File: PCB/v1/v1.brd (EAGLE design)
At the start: 55 x 39 mm, 69 parts, among them U2 AT24C512C-SHD-B

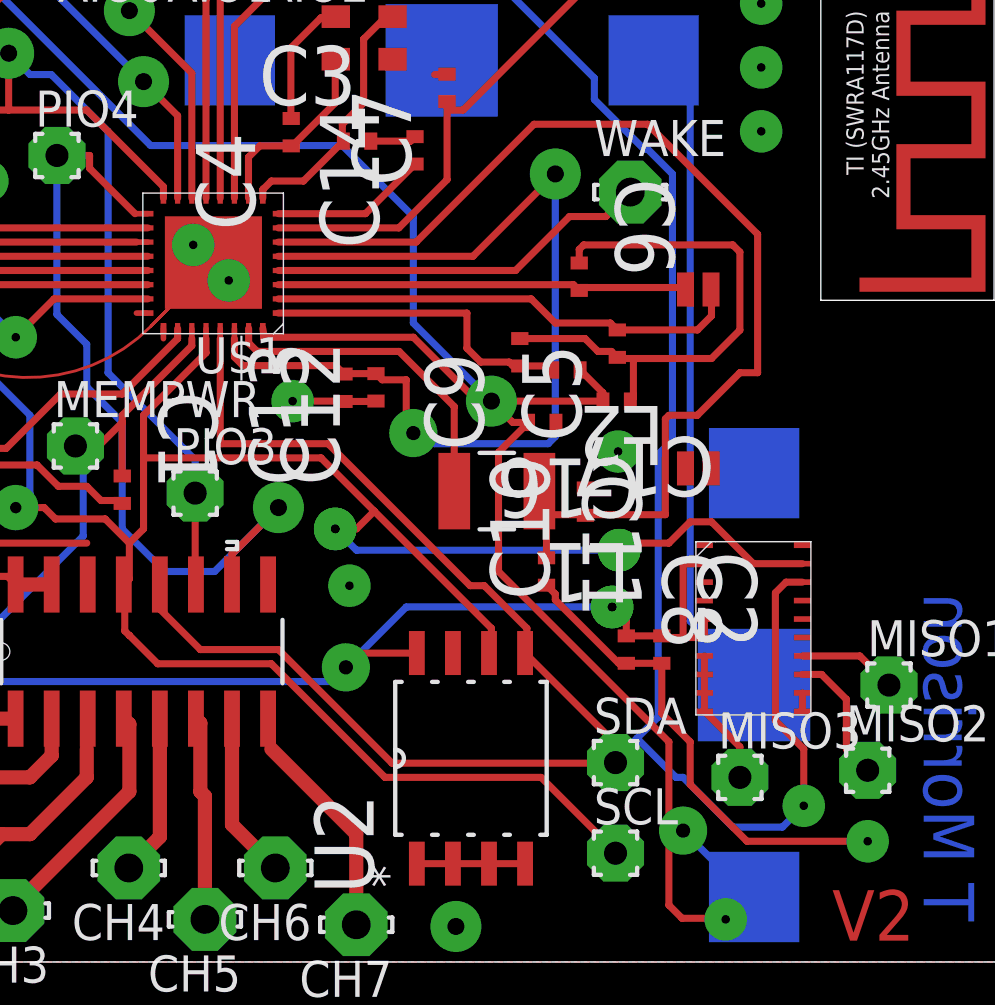
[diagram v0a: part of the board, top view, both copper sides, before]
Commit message: need to check over
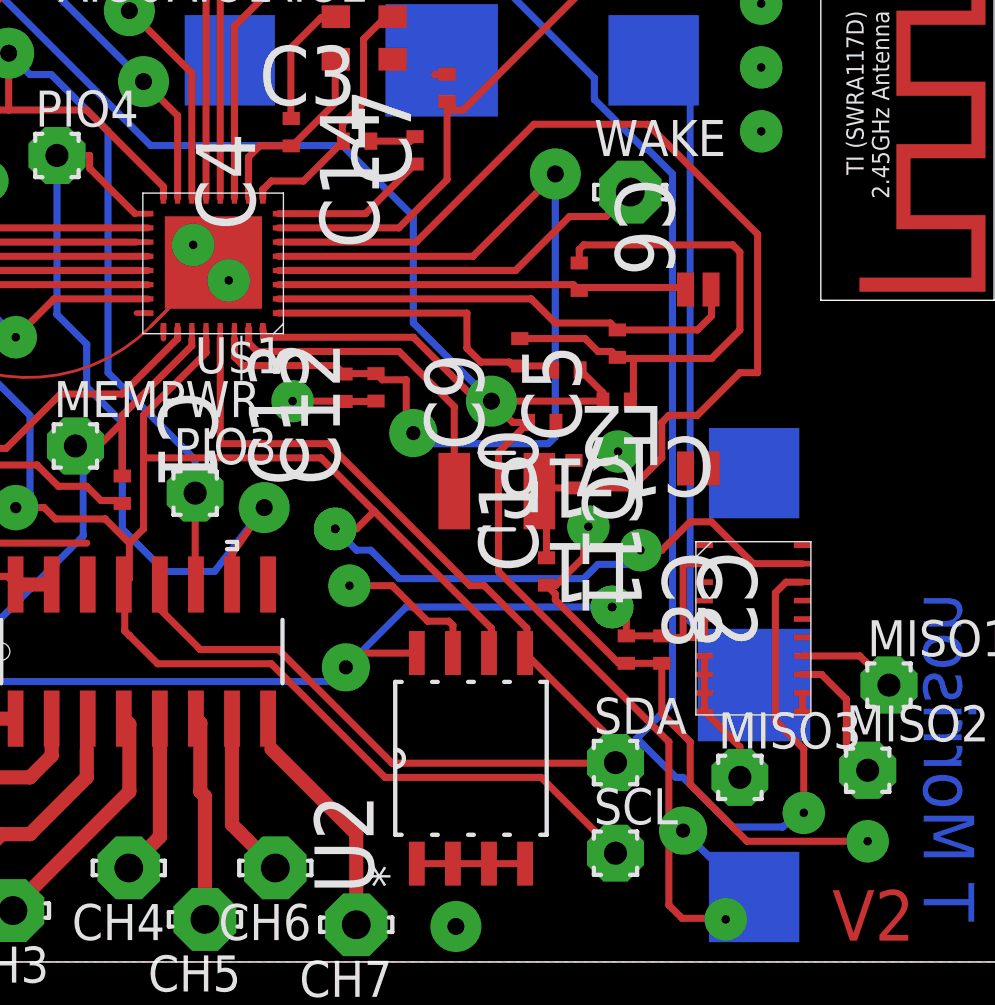
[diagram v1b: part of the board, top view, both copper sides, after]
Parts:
- moved C10 1.05 mm to (39.7, 17.2)
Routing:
- net GND: track 112.2 -> 124.5 mm, vias 11 -> 14
- net N$39: track 40.0 -> 38.7 mm
- net SCL: track 97.6 -> 98.4 mm
- net N$25: track 28.4 -> 27.8 mm
